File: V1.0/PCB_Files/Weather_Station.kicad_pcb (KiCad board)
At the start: 2 copper layers, 44 parts, among them J1 N091-2832TSWFG02-H14, J2 USB_B_Micro, J3 Conn_01x04_Pin, J4 Conn_01x04_Pin, U1 STM32F103C8T6, U2 HDC1080DMBR, U3 AMS1117-3.3, U5 SRV05-4, Y1 X322516MLB4SI

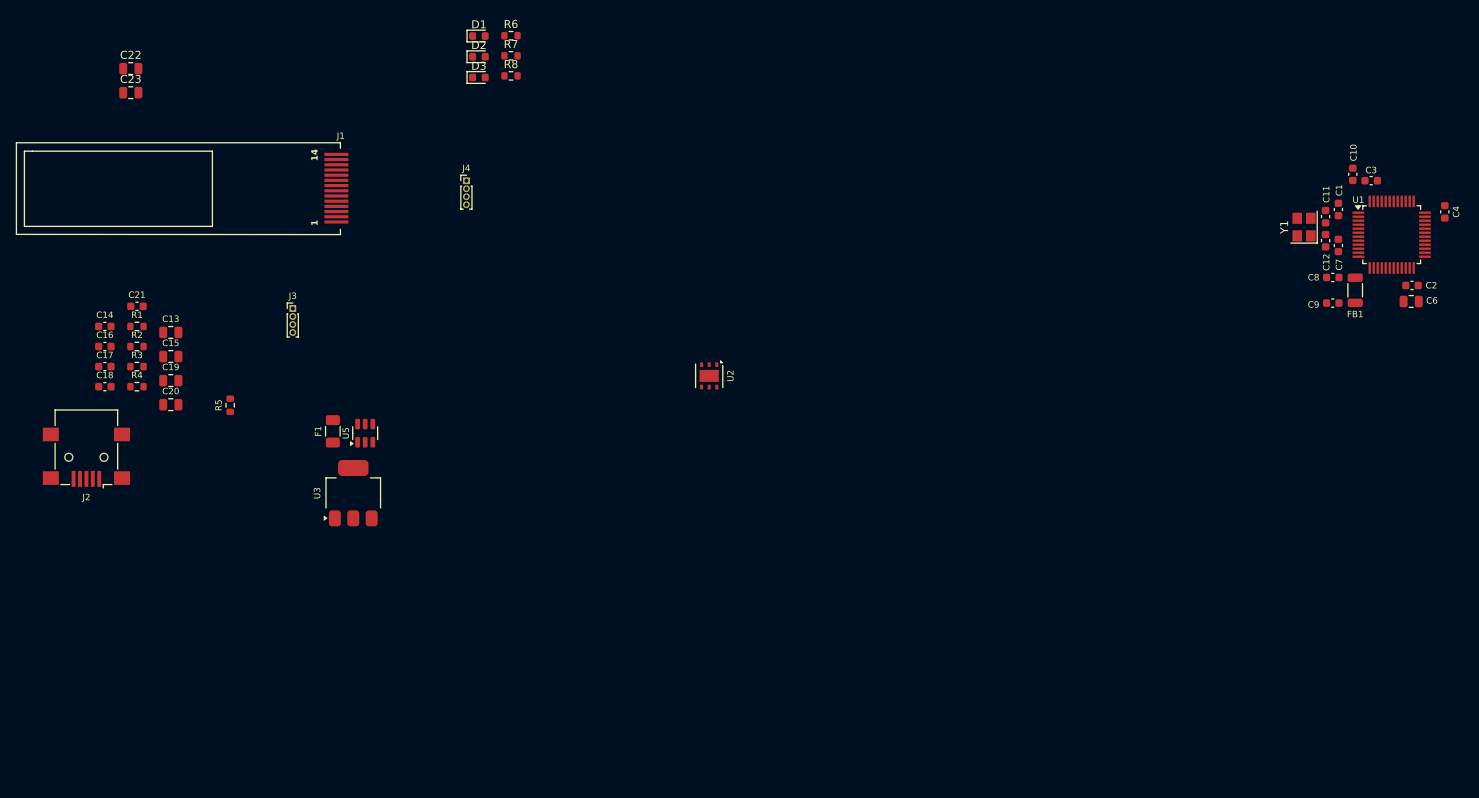
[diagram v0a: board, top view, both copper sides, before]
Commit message: Made Progress with STM32 Layout.
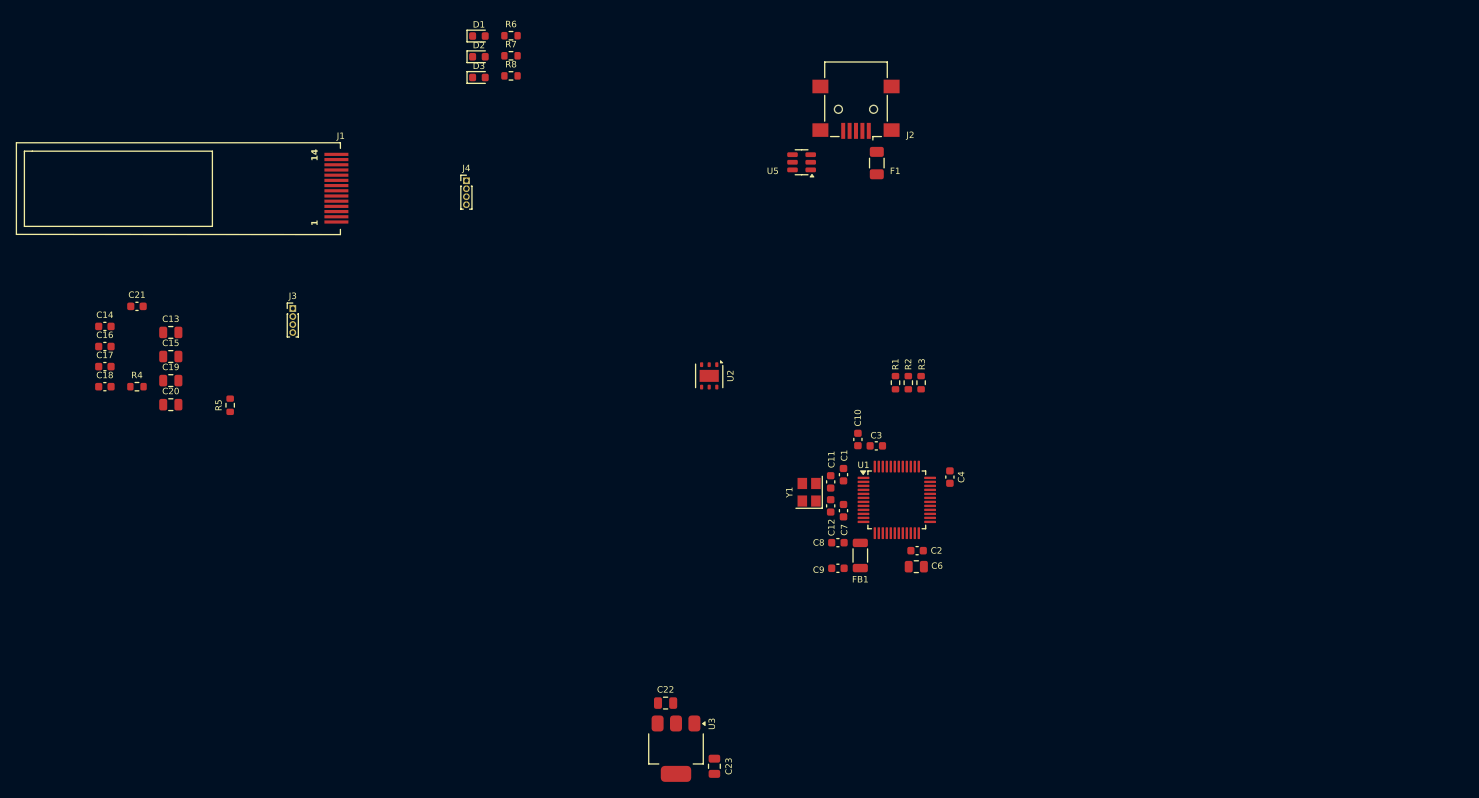
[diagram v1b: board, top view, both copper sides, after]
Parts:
- moved C23 111.4 mm to (142.5, 116.2), turned to 90 degrees
- moved J2 105.6 mm to (160.2, 34.1)
- moved C22 103.7 mm to (136.4, 108.3)
- moved R3 98.0 mm to (168.3, 68.2), turned to -90 degrees
- moved R2 96.5 mm to (166.7, 68.2), turned to -90 degrees
- moved R1 95.1 mm to (165.1, 68.2), turned to -90 degrees
- moved F1 75.8 mm to (162.8, 40.8)
- moved C1 70.2 mm to (158.6, 79.8)
- moved C10 70.2 mm to (160.4, 75.3)
- moved C11 70.2 mm to (157.0, 80.7)
- moved C12 70.2 mm to (157.0, 83.7)
- moved C4 70.2 mm to (171.9, 80.0)
- moved C7 70.2 mm to (158.6, 84.2)
- moved C8 70.2 mm to (157.9, 88.2)
- moved C9 70.2 mm to (157.9, 91.5)
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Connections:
- net /USB_DM renamed /USB_D-
- net /USB_DP renamed /USB_D+
- C22 pad 2: Net-(C22-Pad2) -> GND
- C23 pad 2: Net-(C22-Pad2) -> GND
- F1 pad 2: Net-(J2-VBUS) -> /VBUS_IN
- J2 pad 1: Net-(J2-VBUS) -> /VBUS_IN
- R5 pad 1: Net-(J2-VBUS) -> VBUS
- U5 pad 5: Net-(J2-VBUS) -> VBUS
